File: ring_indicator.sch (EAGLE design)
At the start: 19 parts, among them Q2 BUZ11

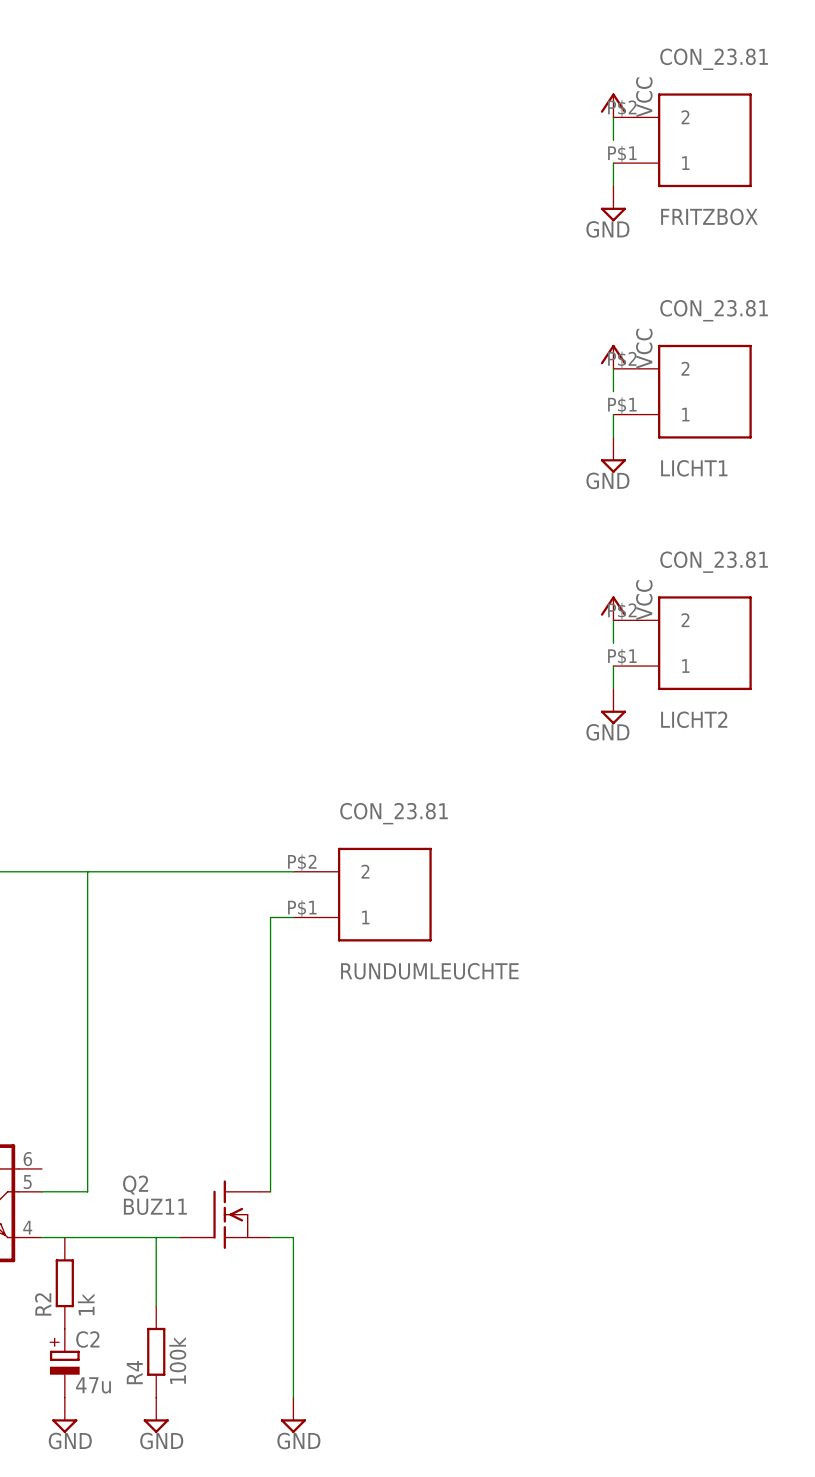
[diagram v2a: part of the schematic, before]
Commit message: v0.2.2-layout simplified
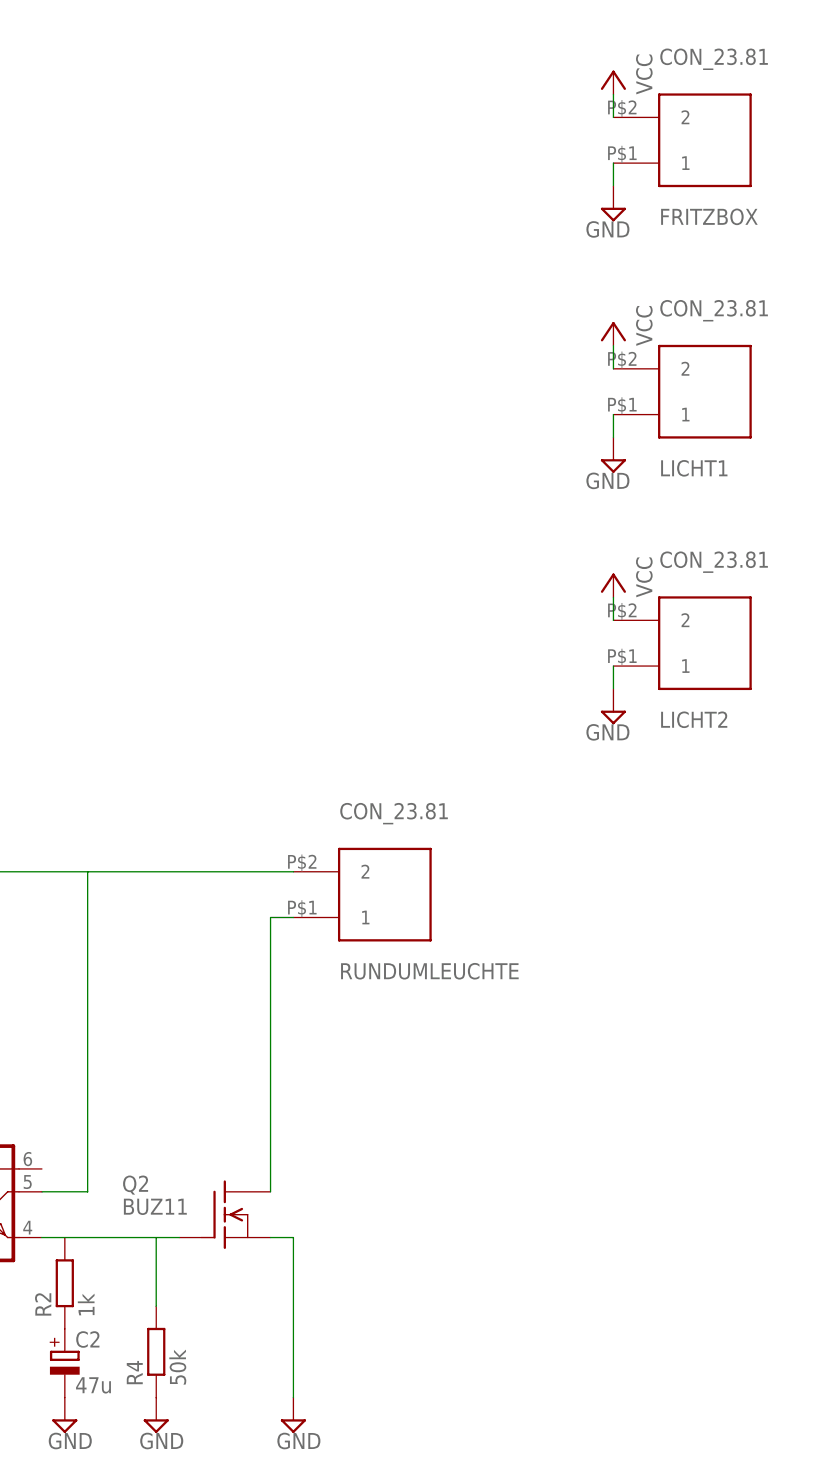
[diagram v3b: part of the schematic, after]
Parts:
- R4: value 100k -> 50k
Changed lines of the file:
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@@
 <part name="R3" library="rcl" deviceset="R-EU_" device="0207/10" value="2k2"/>
 <part name="LED1" library="led" deviceset="LED" device="5MM"/>
-<part name="R4" library="rcl" deviceset="R-EU_" device="0207/10" value="100k"/>
+<part name="R4" library="rcl" deviceset="R-EU_" device="0207/10" value="50k"/>
 <part name="OK1" library="optocoupler" deviceset="4N*?M" device="" technology="27"/>
 <part name="Q2" library="transistor-fet" deviceset="BUZ11" device=""/>
@@
 <instance part="RUNDUMLEUCHTE" gate="G$1" x="220.98" y="33.02" rot="MR180"/>
 <instance part="SUPPLY1" gate="GND" x="246.38" y="109.22" rot="MR0"/>
-<instance part="P+1" gate="VCC" x="246.38" y="121.92" rot="MR0"/>
-<instance part="P+2" gate="VCC" x="246.38" y="93.98" rot="MR0"/>
-<instance part="P+3" gate="VCC" x="246.38" y="66.04" rot="MR0"/>
+<instance part="P+1" gate="VCC" x="246.38" y="124.46" rot="MR0"/>
+<instance part="P+2" gate="VCC" x="246.38" y="96.52" rot="MR0"/>
+<instance part="P+3" gate="VCC" x="246.38" y="68.58" rot="MR0"/>
 <instance part="SUPPLY2" gate="GND" x="246.38" y="81.28" rot="MR0"/>
 <instance part="SUPPLY3" gate="GND" x="246.38" y="53.34" rot="MR0"/>
@@
 <segment>
 <pinref part="FRITZBOX" gate="G$1" pin="2"/>
-<wire x1="246.38" y1="116.84" x2="246.38" y2="119.38" width="0.1524" layer="91"/>
 <pinref part="P+1" gate="VCC" pin="VCC"/>
+<wire x1="246.38" y1="121.92" x2="246.38" y2="119.38" width="0.1524" layer="91"/>
 </segment>
 <segment>
 <pinref part="LICHT1" gate="G$1" pin="2"/>
-<wire x1="246.38" y1="88.9" x2="246.38" y2="91.44" width="0.1524" layer="91"/>
 <pinref part="P+2" gate="VCC" pin="VCC"/>
+<wire x1="246.38" y1="93.98" x2="246.38" y2="91.44" width="0.1524" layer="91"/>
 </segment>
 <segment>
 <pinref part="LICHT2" gate="G$1" pin="2"/>
-<wire x1="246.38" y1="60.96" x2="246.38" y2="63.5" width="0.1524" layer="91"/>
 <pinref part="P+3" gate="VCC" pin="VCC"/>
+<wire x1="246.38" y1="66.04" x2="246.38" y2="63.5" width="0.1524" layer="91"/>
 </segment>
 <segment>
